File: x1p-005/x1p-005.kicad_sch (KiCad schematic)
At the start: 41 parts, among them Q1 LMBT3904LT1G, SW1 6.0*6.0*6.0, SW2 6.0*6.0*6.0, U1 AD24C02, U2 SN74LVC1T45DBVR, U4 SN74LVC1G3157DBVR_C3040658, U5 SN74LVC1G3157DBVR_C3040658

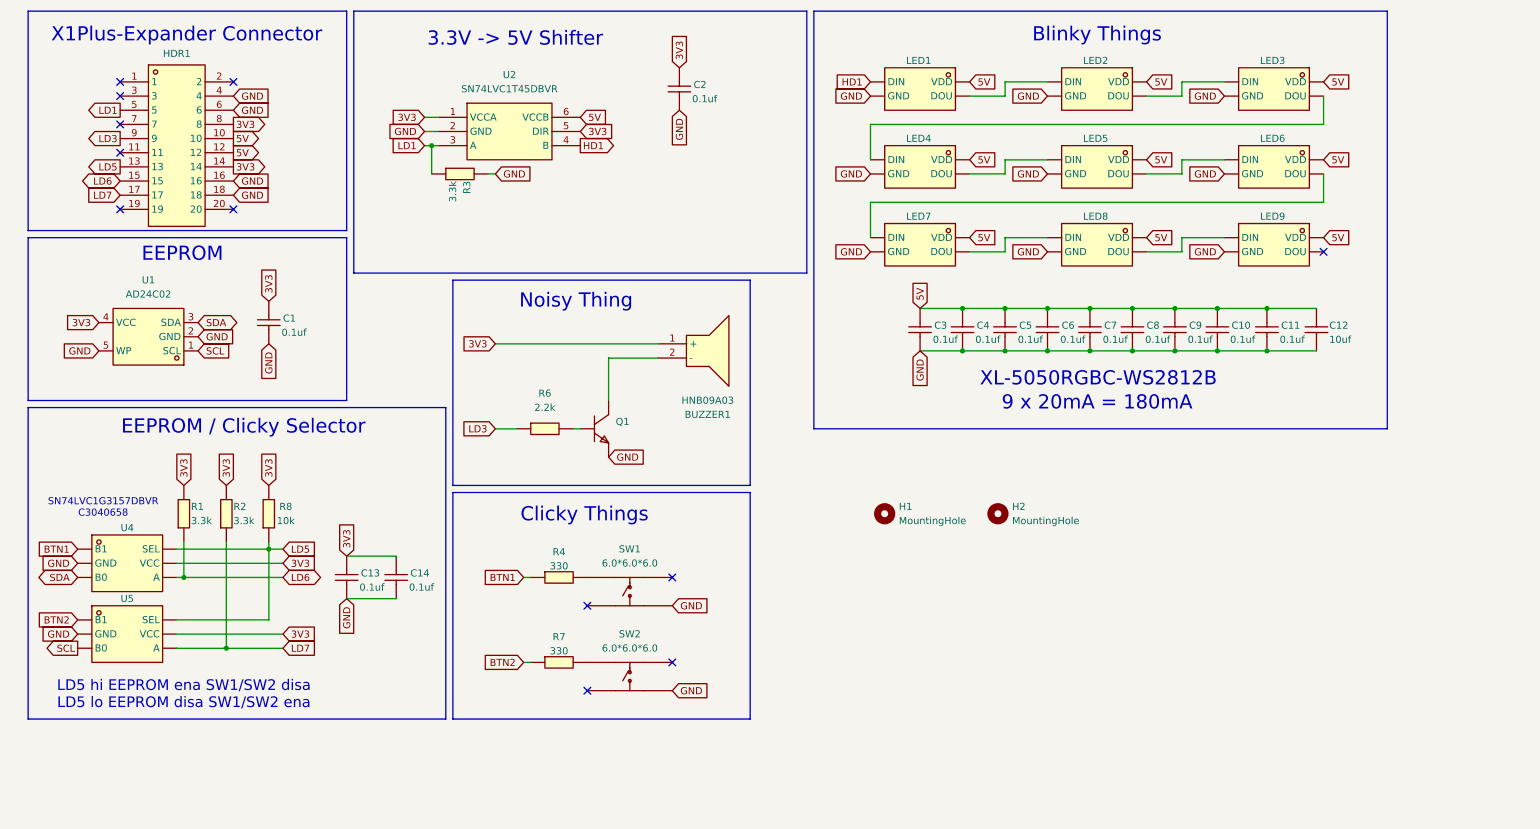
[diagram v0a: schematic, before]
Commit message: x1p-005-b01-fixes-1
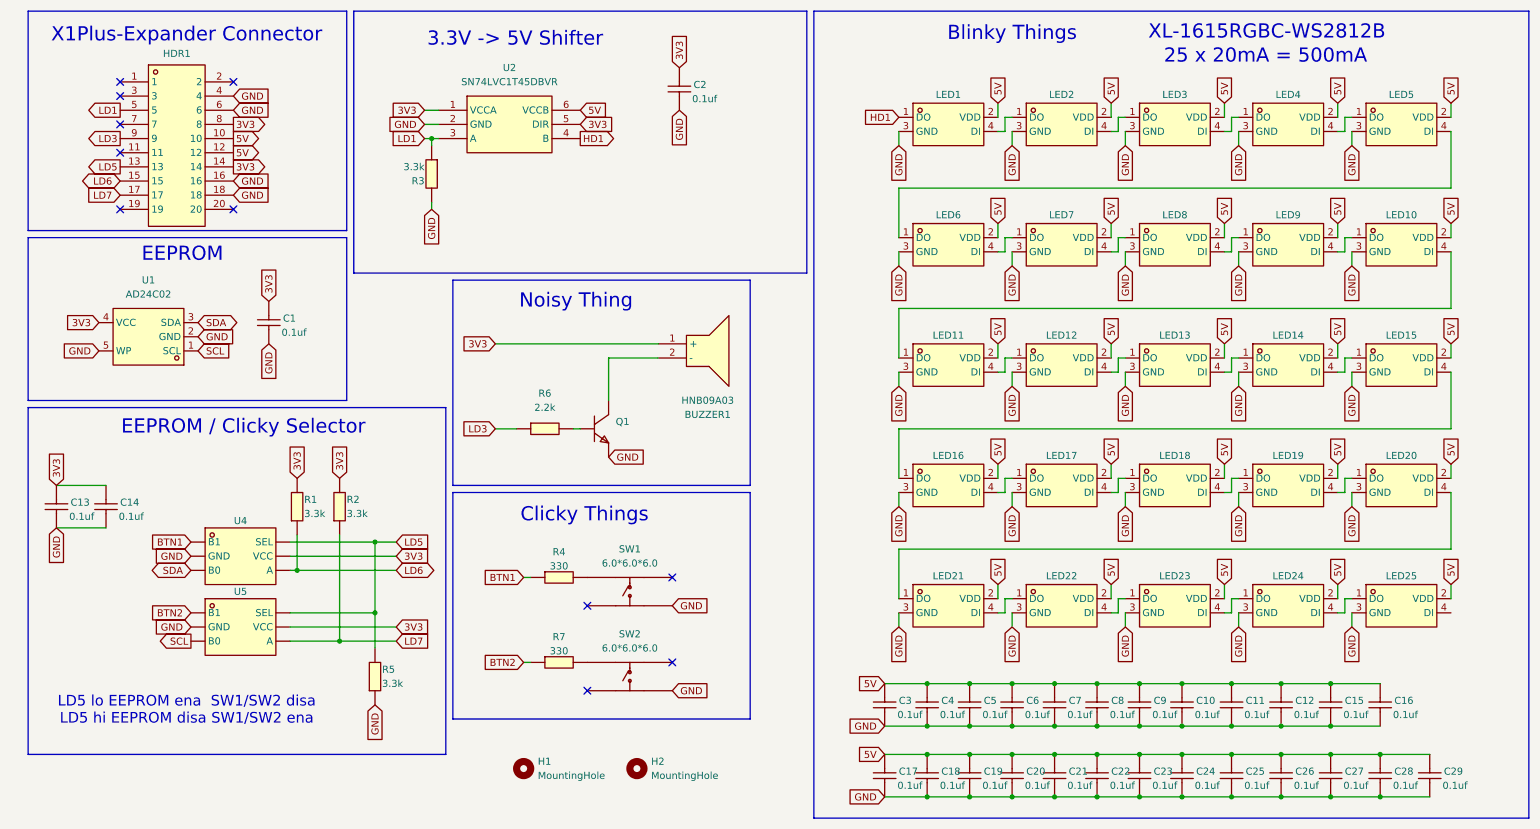
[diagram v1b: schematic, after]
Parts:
- removed C12: 10uf, x1p-005:C1206, symbol x1p-005:CL31A106KBHNNNE
- removed LED1, LED2, LED3, LED4, LED5, LED6, LED7, LED8, LED9: XL-5050RGBC-WS2812B, x1p-005:LED-SMD_4P-L5.0-W5.0-BL_XL-5050RGBC, symbol x1p-005:XL-5050RGBC-WS2812B
- removed R8: 10k, x1p-005:R0402, symbol x1p-005:0402WGF1002TCE
- added C12, C15, C16, C17, C18, C19, C20, C21, C22, C23, C24, C25, C26, C27, C28, C29: 0.1uf, x1p-004:C0402, symbol lcsc:CL05B104KO5NNNC
- added LED1, LED10, LED11, LED12, LED13, LED14, LED15, LED16, LED17, LED18, LED19, LED2, LED20, LED21, LED22, LED23, LED24, LED25, LED3, LED4, LED5, LED6, LED7, LED8, LED9: XL-1615RGBC-WS2812B, x1p-005:LED-SMD_4P-L1.6-W1.5_XL-1615RGBC-WS2812B, symbol x1p-005:XL-1615RGBC-WS2812B
- added R5: 3.3k, x1p-005:R0402, symbol lcsc:0402WGF3301TCE
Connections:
- net 5V: now also C12.1, C15.1, C16.1, C17.1, C18.1, C19.1, C20.1, C21.1, C22.1, C23.1, C24.1, C25.1, C26.1, C27.1, C28.1, C29.1, LED1.2 (VDD), LED10.2 (VDD), LED11.2 (VDD), LED12.2 (VDD), LED13.2 (VDD), LED14.2 (VDD), LED15.2 (VDD), LED16.2 (VDD), LED17.2 (VDD), LED18.2 (VDD), LED19.2 (VDD), LED2.2 (VDD), LED20.2 (VDD), LED21.2 (VDD), LED22.2 (VDD), LED23.2 (VDD), LED24.2 (VDD), LED25.2 (VDD), LED3.2 (VDD), LED4.2 (VDD), LED5.2 (VDD), LED6.2 (VDD), LED7.2 (VDD), LED8.2 (VDD), LED9.2 (VDD)
- net GND: now also C12.2, C15.2, C16.2, C17.2, C18.2, C19.2, C20.2, C21.2, C22.2, C23.2, C24.2, C25.2, C26.2, C27.2, C28.2, C29.2, LED1.3 (GND), LED10.3 (GND), LED11.3 (GND), LED12.3 (GND), LED13.3 (GND), LED14.3 (GND), LED15.3 (GND), LED16.3 (GND), LED17.3 (GND), LED18.3 (GND), LED19.3 (GND), LED2.3 (GND), LED20.3 (GND), LED21.3 (GND), LED22.3 (GND), LED23.3 (GND), LED24.3 (GND), LED25.3 (GND), LED3.3 (GND), LED4.3 (GND), LED5.3 (GND), LED6.3 (GND), LED7.3 (GND), LED8.3 (GND), LED9.3 (GND), R5.1
- net HD1: now also LED1.1 (DO)
- net LD5: now also R5.2
- new net: LED16.4 (DI), LED17.1 (DO)
- new net: LED17.4 (DI), LED18.1 (DO)
- new net: LED1.4 (DI), LED2.1 (DO)
- new net: LED15.4 (DI), LED16.1 (DO)
- new net: LED24.4 (DI), LED25.1 (DO)
- new net: LED6.4 (DI), LED7.1 (DO)
- new net: LED7.4 (DI), LED8.1 (DO)
- new net: LED4.4 (DI), LED5.1 (DO)
- new net: LED5.4 (DI), LED6.1 (DO)
- new net: LED12.4 (DI), LED13.1 (DO)
- new net: LED13.4 (DI), LED14.1 (DO)
- new net: LED18.4 (DI), LED19.1 (DO)
- new net: LED10.1 (DO), LED9.4 (DI)
- new net: LED10.4 (DI), LED11.1 (DO)
- new net: LED3.4 (DI), LED4.1 (DO)
- new net: LED19.4 (DI), LED20.1 (DO)
- new net: LED14.4 (DI), LED15.1 (DO)
- new net: LED22.4 (DI), LED23.1 (DO)
- new net: LED23.4 (DI), LED24.1 (DO)
- new net: LED20.4 (DI), LED21.1 (DO)
- new net: LED21.4 (DI), LED22.1 (DO)
- new net: LED11.4 (DI), LED12.1 (DO)
- new net: LED8.4 (DI), LED9.1 (DO)
- new net: LED2.4 (DI), LED3.1 (DO)
- no-connect marks 12 -> 11
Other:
- note added: "25 x 20mA = 500mA"
- note added: "LD5 lo EEPROM ena SW1/SW2 disa LD5 hi EEPROM disa SW1/SW2 ena"
- note added: "XL-1615RGBC-WS2812B"
- note removed: "9 x 20mA = 180mA"
- note removed: "LD5 hi EEPROM ena SW1/SW2 disa LD5 lo EEPROM disa SW1/SW2 ena"
- note removed: "SN74LVC1G3157DBVR C3040658"
- note removed: "XL-5050RGBC-WS2812B"
- moved on the sheet: C13, C14, R1, R2, R3, U2, U4, U5
